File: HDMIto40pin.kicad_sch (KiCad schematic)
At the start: 56 parts, among them J17 TTL 40Pin, J18 I2C EDID, U11 LM1117DT-3.3, U12 FAN5333BSX, U13 TFP401APZPR, U14 24LC02BT-E/LT

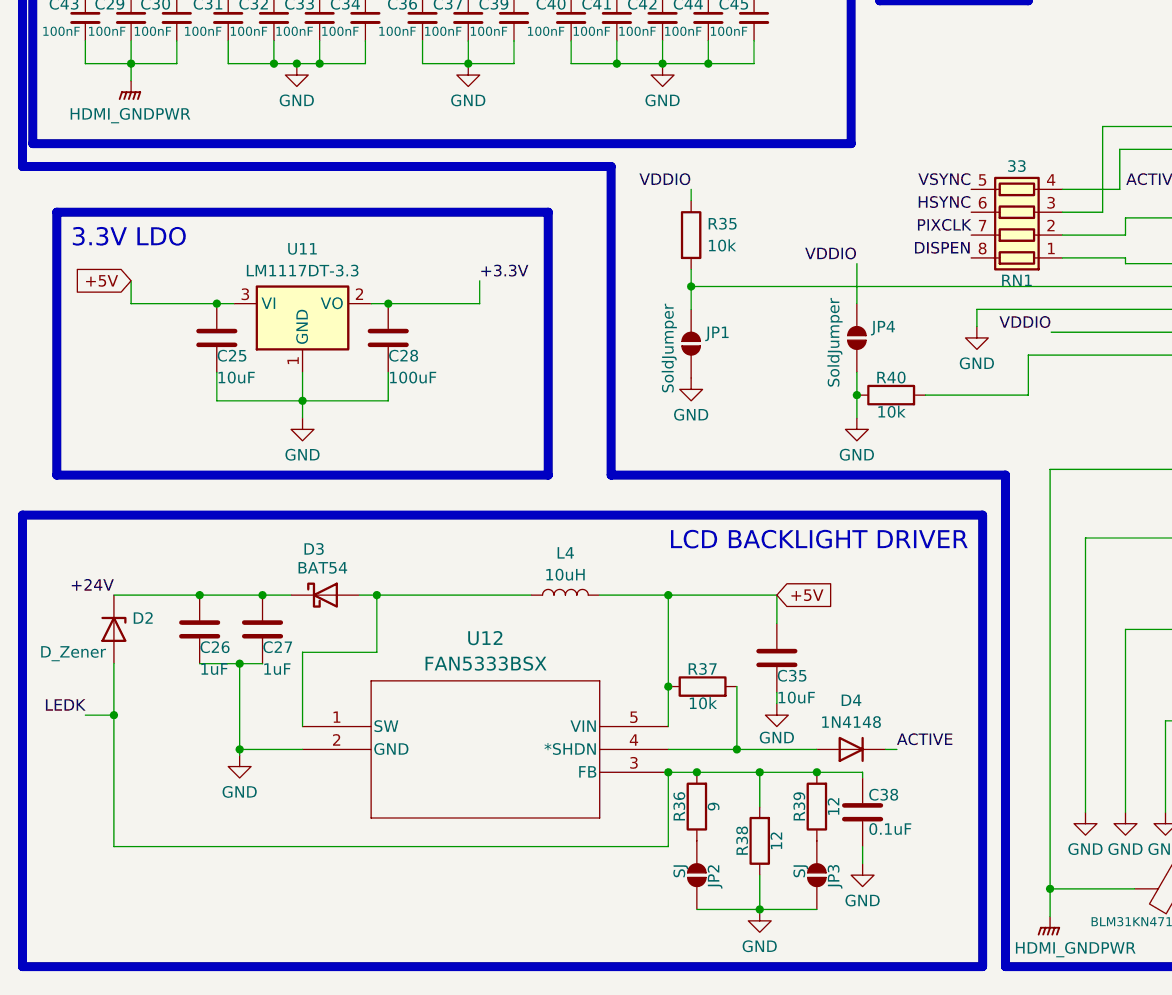
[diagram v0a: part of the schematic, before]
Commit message: update zip
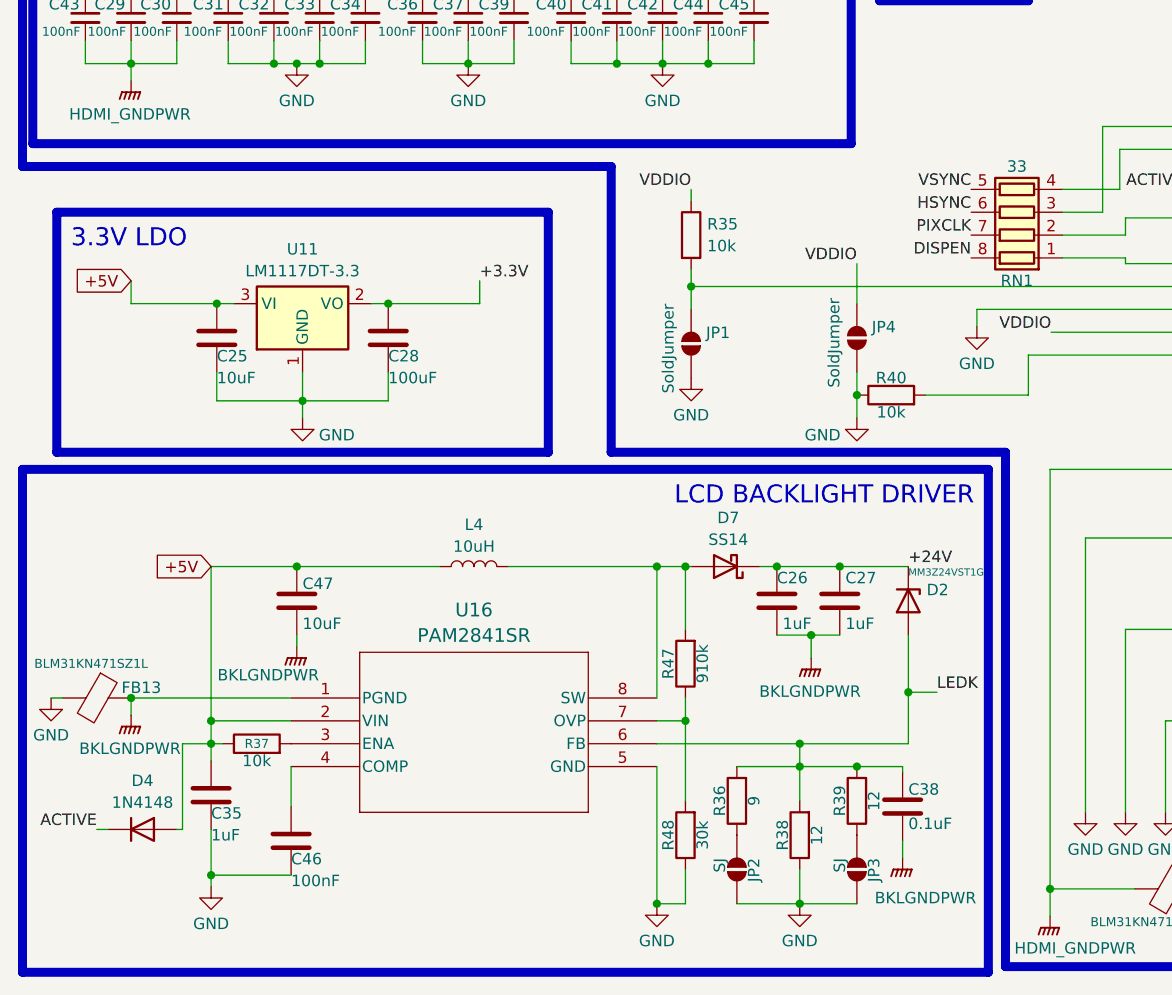
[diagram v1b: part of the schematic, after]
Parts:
- removed D3: BAT54, Package_TO_SOT_SMD:TSOT-23_HandSoldering, symbol Device:D_Schottky
- removed U12: FAN5333BSX, FAN5333:SOT-23-5_ONS, symbol FAN5333:FAN5333BSX
- added C46: 100nF, Capacitor_SMD:C_0603_1608Metric_Pad1.08x0.95mm_HandSolder, symbol Device:C
- added C47: 10uF, Capacitor_SMD:C_0603_1608Metric_Pad1.08x0.95mm_HandSolder, symbol Device:C
- added D7: SS14, Diode_SMD:D_SMA, symbol Diode:SS14
- added FB13: BLM31KN471SZ1L, Inductor_SMD:L_1206_3216Metric_Pad1.22x1.90mm_HandSolder, symbol Device:FerriteBead
- added R47: 910k, Resistor_SMD:R_0603_1608Metric_Pad0.98x0.95mm_HandSolder, symbol Device:R
- added R48: 30k, Resistor_SMD:R_0603_1608Metric_Pad0.98x0.95mm_HandSolder, symbol Device:R
- added U16: PAM2841SR, PAM2841:PAM2841, symbol PAM2841:PAM2841SR
- C35: value 10uF -> 1uF
- D2: value D_Zener -> MM3Z24VST1G
- J17: footprint Connector_FFC-FPC:TE_4-1734839-0_1x40-1MP_P0.5mm_Horizontal -> Connector_FFC-FPC:Omron_XF2M-4015-1A_1x40-1MP_P0.5mm_Horizontal
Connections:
- net +24V: now also D7.1 (K)
- net +5V: now also D4.2 (A), L4.1, C47.1, U16.2 (VIN); no longer L4.2
- net GND: now also C46.2, FB13.2, R48.1, U16.5 (GND); no longer C26.2, C27.2, C38.2
- net LEDK: now also U16.6 (FB)
- net at R37.2: now also U16.3 (ENA); no longer D4.2 (A)
- new net: C46.1, U16.4 (COMP)
- new net: R47.1, R48.2, U16.7 (OVP)
- new net: D7.2 (A), L4.2, R47.2, U16.8 (SW)
- new net BKLGNDPWR: C26.2, C27.2, C38.2, C47.2, FB13.1, U16.1 (PGND)
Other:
- moved on the sheet: C26, C27, C35, C38, D2, D4, JP2, JP3, L4, R36, R37, R38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
